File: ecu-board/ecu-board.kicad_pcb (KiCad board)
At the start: 2 copper layers, 180 x 127.5 mm, 53 parts, among them J1 MicroSquirt_connector, J10 Injector connector, J11 Cockpit connector, J12 EGO connector, J13 Chrankshaft Hall connector, J14 Camshaft Hall connector, J15 Ignition 1 connector, J16 Ignition 2 connector, J17 Camera connector, J18 Wheel Hall connector, J19 Speed sensor connector, J2 Battery power conenctor, J20 CAN connector, J3 MS_breakout_conn, J4 Motor connector, J5 Serial DB9 connector, J6 Controller connector, J7 Backlight connector, J8 IAT connector, J9 CLT connector, K1 Main power relay, K2 Start motor relay, U1 MAP Sensor

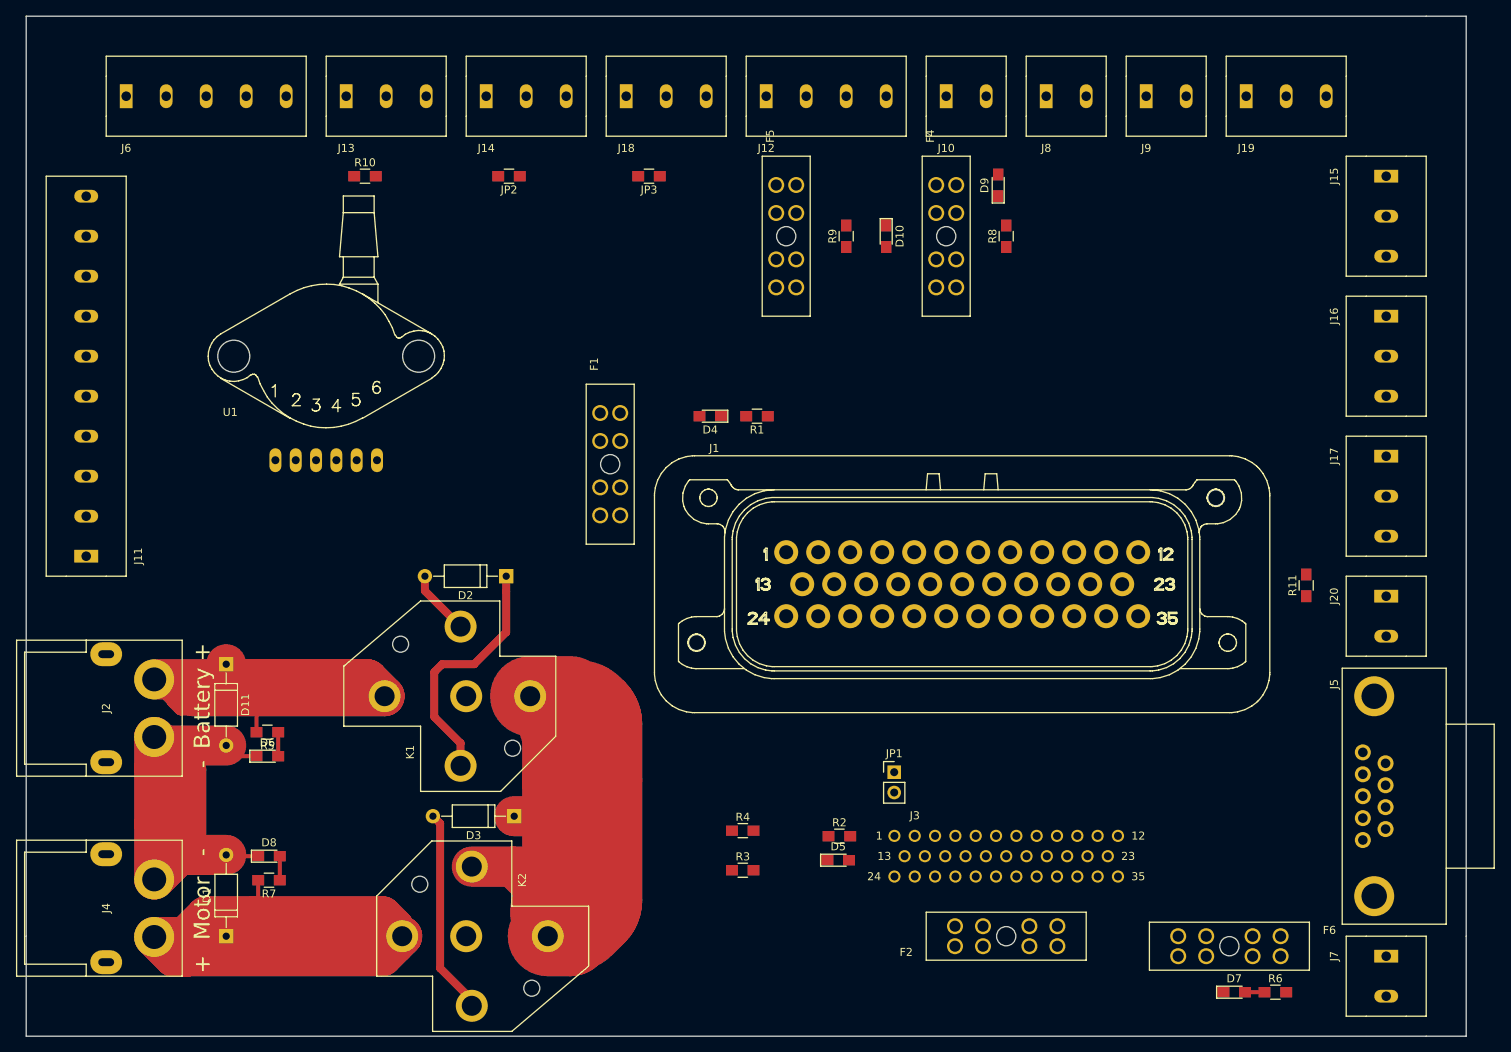
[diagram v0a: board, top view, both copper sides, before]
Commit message: Route almost everything.
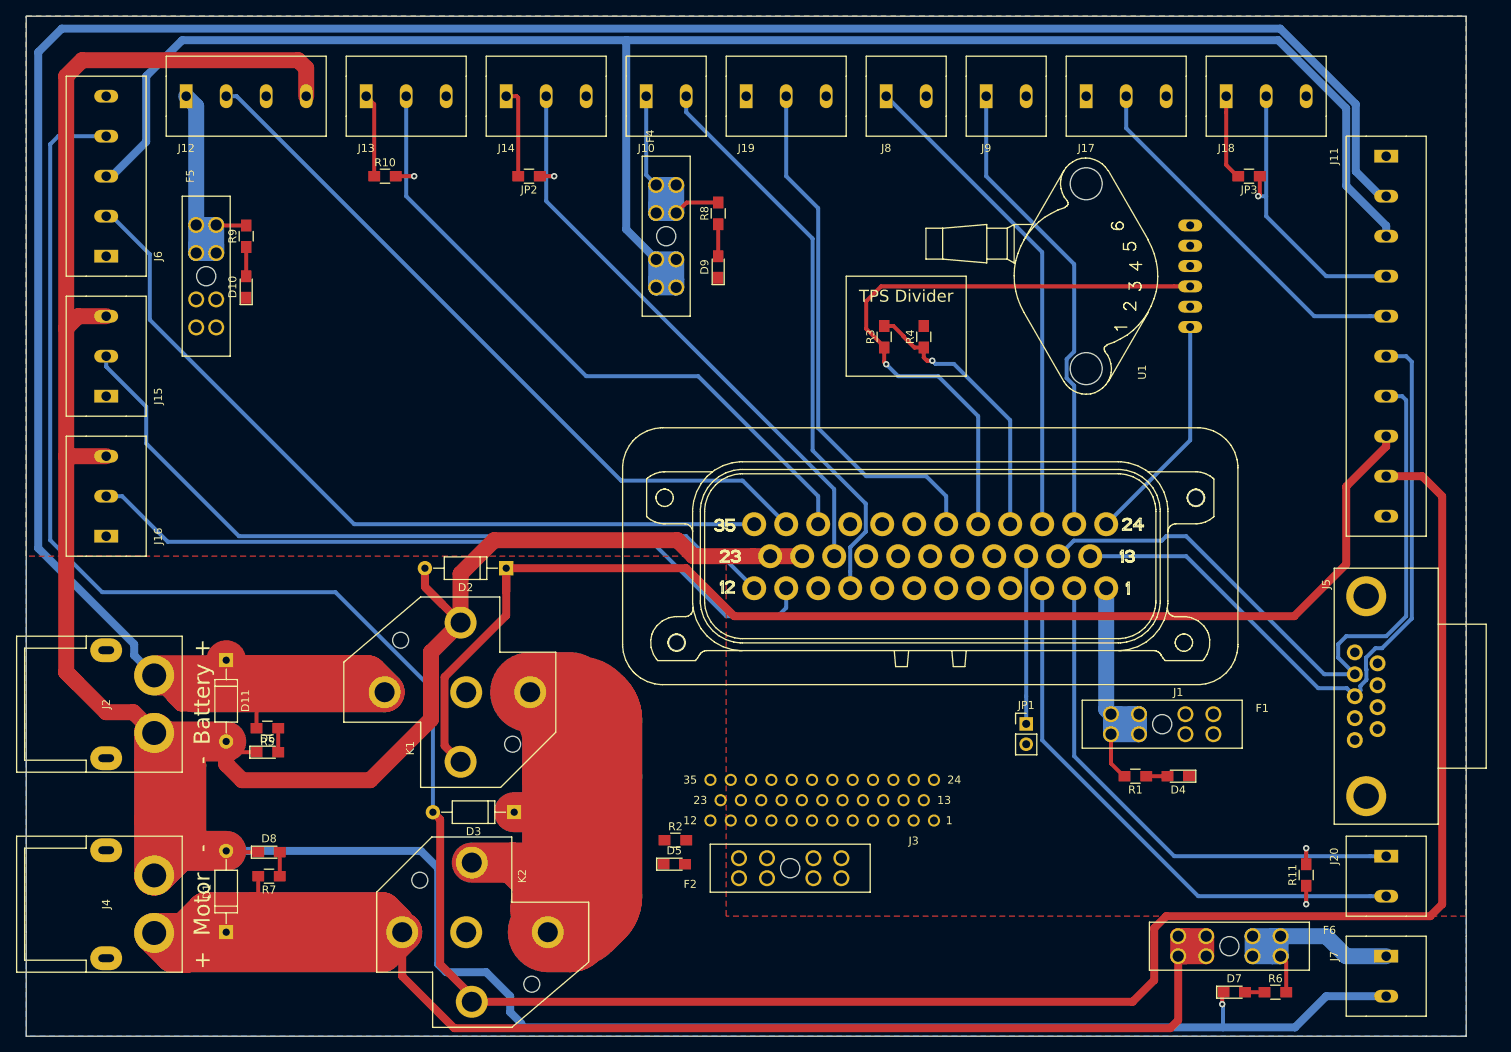
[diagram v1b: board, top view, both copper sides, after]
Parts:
- moved J11 170.0 mm to (220.0, 52.5), turned to 270 degrees
- moved J15 162.3 mm to (60.0, 82.5), turned to 90 degrees
- moved J16 162.3 mm to (60.0, 100.0), turned to 90 degrees
- moved U1 95.5 mm to (182.5, 67.5), turned to 90 degrees
- moved D10 80.3 mm to (77.5, 68.8), turned to 90 degrees
- moved F1 76.3 mm to (192.0, 123.5), turned to 0 degrees
- moved J18 75.0 mm to (200.0, 45.0)
- moved JP3 75.0 mm to (202.8, 55.0)
- moved R9 75.0 mm to (77.5, 62.5)
- moved D4 73.8 mm to (194.0, 130.0)
- moved F5 72.7 mm to (72.5, 67.5)
- moved J12 72.5 mm to (70.0, 45.0)
- moved R3 69.0 mm to (157.2, 75.1), turned to 90 degrees
- moved R4 65.7 mm to (162.2, 75.1), turned to 90 degrees
- moved R1 65.3 mm to (188.7, 130.0)
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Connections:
- D2 pad 2: GNDS -> GNDPWR
- K1 pad 85: GNDS -> GNDPWR
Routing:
- net GNDPWR: track 125.0 -> 538.2 mm, vias 0 -> 1
- net /button_to_start_motor_relay: track 25.7 -> 342.7 mm
- net +BATT: track 168.6 -> 435.8 mm
- net /Connectors/deadmans: track 0.00 -> 238.5 mm
- net /relay_to_start_motor: track 183.7 -> 318.4 mm
- net /button_to_main_relay: track 31.1 -> 159.4 mm
- net /tachometer: track 0.00 -> 101.8 mm
- net /ignition_1: track 0.00 -> 96.5 mm
- net /ignition_2: track 0.00 -> 94.1 mm
- net /ego_signal: track 0.00 -> 92.2 mm
- net /serial_TX: track 0.00 -> 89.5 mm
- net /serial_RX: track 0.00 -> 89.1 mm
- net /crank_hall_signal: track 0.00 -> 86.3 mm, vias 0 -> 1
- net +5V: track 0.00 -> 77.9 mm, vias 0 -> 1
- net /cam_hall_signal: track 0.00 -> 75.2 mm, vias 0 -> 1
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- added copper zone on B.Cu, net +12V
- added copper zone on F.Cu, net GNDS
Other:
- outline, holes or cut-outs redrawn
- board text added: "TPS Divider"
